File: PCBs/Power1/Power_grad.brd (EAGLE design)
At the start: 80.9 x 67.1 mm, 21 parts

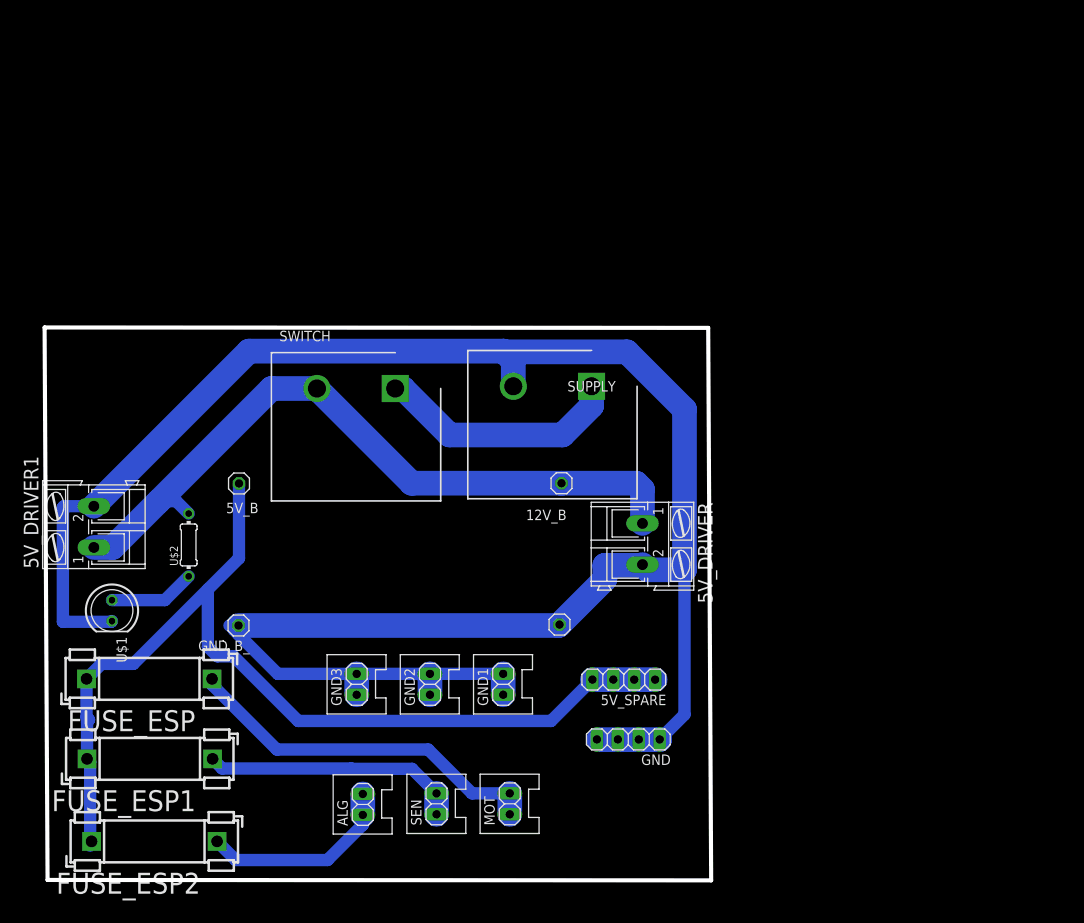
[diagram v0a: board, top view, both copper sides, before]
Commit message: Power modify
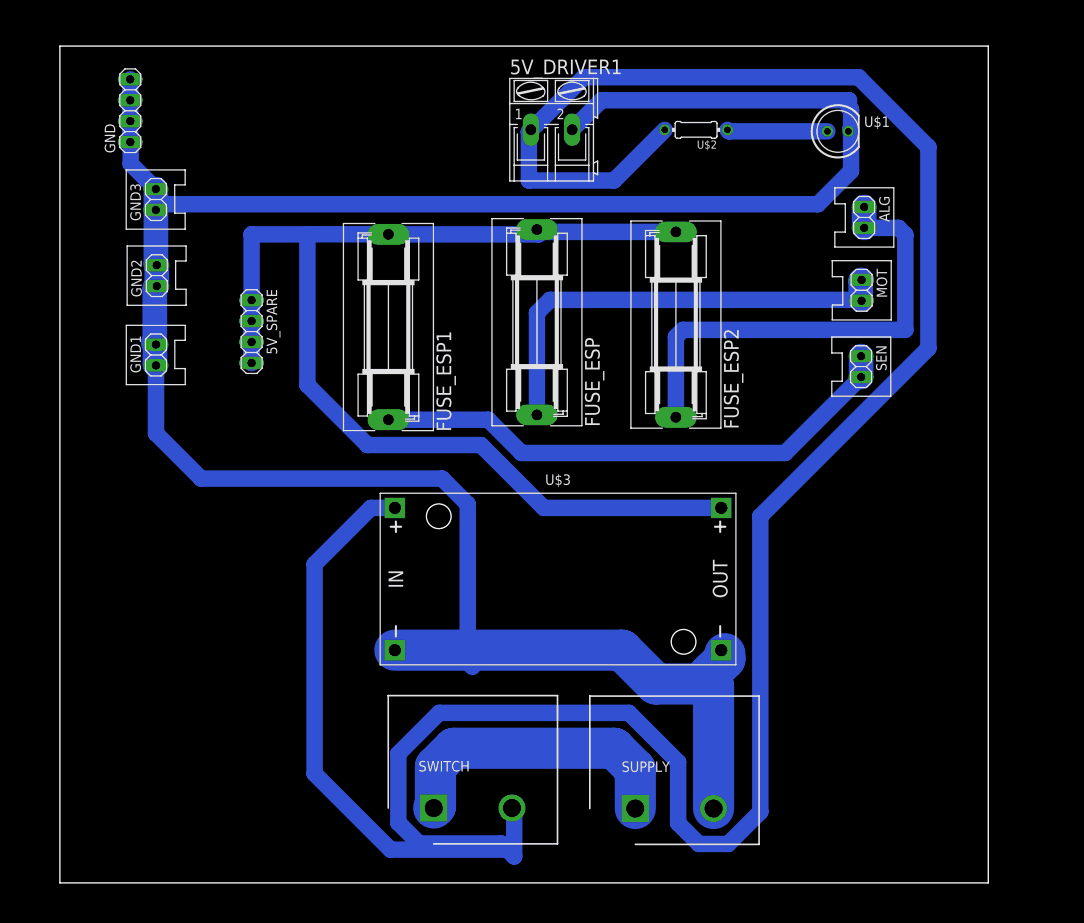
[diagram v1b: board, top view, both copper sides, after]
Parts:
- removed 12V_B, 5V_B, GND_B, GND_B_: (no value), ALL:1X01
- removed 5V_DRIVER: (no value), ALL:AK300/2
- added U$3: DC-DC-STEP-DOWN-LM2596, ALL:DC-DC-STEP-DOWN-LM2596
- FUSE_ESP, FUSE_ESP1, FUSE_ESP2: value FUSEBLANK_5X20MM -> (none); device fuse:FUSE_HOLDER_5X20MM -> ALL:SH22,5A
- moved U$1 105.6 mm to (94.4, 91.2), turned to 0 degrees
- moved GND 97.4 mm to (8.54, 93.7), turned to 90 degrees
- moved ALG 93.7 mm to (97.6, 80.8), turned to 270 degrees
- moved FUSE_ESP2 83.9 mm to (74.8, 67.8), turned to 90 degrees
- moved U$2 79.6 mm to (77.2, 91.4), turned to 180 degrees
- moved MOT 75.6 mm to (97.3, 71.9), turned to 270 degrees
- moved SEN 74.0 mm to (97.3, 62.7), turned to 270 degrees
- moved 5V_DRIVER1 73.6 mm to (59.7, 91.4), turned to 0 degrees
- moved GND3 63.7 mm to (11.7, 83.0)
- moved 5V_SPARE 61.9 mm to (23.3, 66.9), turned to 270 degrees
- moved GND2 59.7 mm to (11.8, 73.7)
- moved FUSE_ESP 58.6 mm to (57.9, 68.1), turned to 90 degrees
- moved GND1 58.1 mm to (11.7, 64.1)
- moved FUSE_ESP1 56.6 mm to (39.9, 67.5), turned to 90 degrees
- moved SUPPLY 51.5 mm to (69.8, 9.03), turned to 0 degrees
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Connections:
- net 12V: now also U$3.IN+; no longer 12V_B.1, 5V_DRIVER.1
- net 5V: now also U$3.OUT+; no longer 5V_B.1
- net GND: now also U$3.IN-, U$3.OUT-; no longer 5V_DRIVER.2, GND_B.1, GND_B_.1
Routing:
- net 12V: track 88.0 -> 323.1 mm
- net SEN: track 31.5 -> 65.4 mm
- net GND: track 263.2 -> 296.5 mm
- net ALG: track 24.1 -> 57.4 mm
- net 5V: track 121.6 -> 150.1 mm
- net MOT: track 44.9 -> 55.0 mm
- net 12V_IN: track 30.0 -> 36.1 mm
- net N$1: track 10.5 -> 12.2 mm
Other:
- board size 80.9 x 67.1 mm -> 112.7 x 101.6 mm

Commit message: PID v1.0
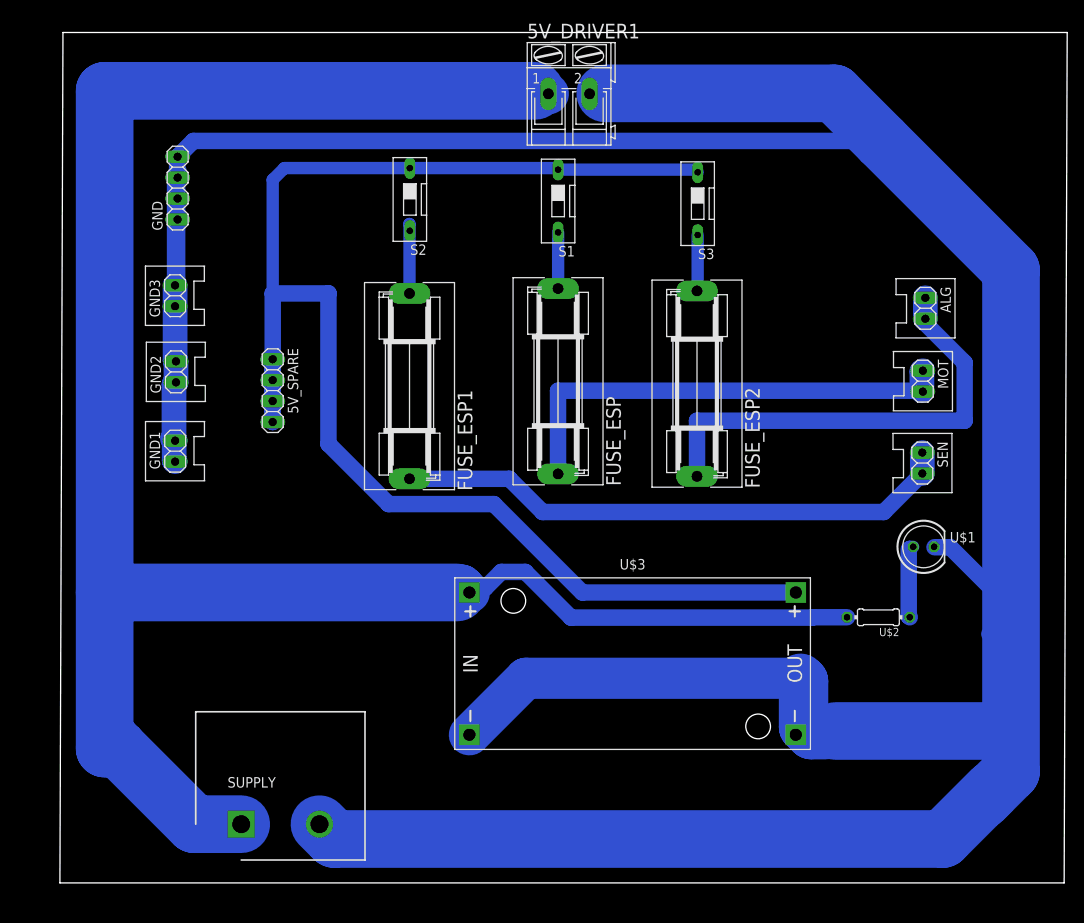
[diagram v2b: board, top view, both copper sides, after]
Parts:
- removed SWITCH: HB9500-9.5-2P, HB9500-9.5-2P:SHDR2W140P0X950_1X2_2055X1800X
- added S1, S2, S3: (no value), ALL:DS-01
- moved U$2 63.2 mm to (99.4, 32.2)
- moved U$1 51.5 mm to (104.8, 40.8)
- moved SUPPLY 47.9 mm to (22.0, 7.13)
- moved SEN 13.9 mm to (104.7, 51.0)
- moved U$3 13.7 mm to (69.5, 26.6)
- moved ALG 13.3 mm to (105.1, 69.8)
- moved MOT 13.3 mm to (104.8, 60.9)
- moved GND1 11.9 mm to (14.0, 52.4)
- moved GND2 11.9 mm to (14.1, 62.0)
- moved GND3 11.9 mm to (14.0, 71.3)
- moved GND 11.0 mm to (14.3, 84.3)
- moved 5V_SPARE 7.61 mm to (25.8, 59.8)
- moved FUSE_ESP2 7.61 mm to (77.3, 60.6)
- moved FUSE_ESP1 7.61 mm to (42.4, 60.3)
- moved FUSE_ESP 7.61 mm to (60.5, 60.9)
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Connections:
- removed net 12V_IN: SUPPLY.1, SWITCH.1
- new net N$2: FUSE_ESP1.2, S2.2
- new net N$3: FUSE_ESP.2, S1.2
- new net N$4: FUSE_ESP2.2, S3.2
- net 12V: now also SUPPLY.1; no longer SWITCH.2
- net 5V: now also S1.1, S2.1, S3.1; no longer FUSE_ESP.2, FUSE_ESP1.2, FUSE_ESP2.2
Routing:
- net GND: track 296.5 -> 454.6 mm
- net 12V: track 323.1 -> 264.1 mm
- net 12V_IN: track 36.1 -> 0.00 mm
- net 5V: track 150.1 -> 178.7 mm
- net N$2: track 0.00 -> 8.45 mm
- net N$3: track 0.00 -> 6.82 mm
- net N$4: track 0.00 -> 6.82 mm
- net N$1: track 12.2 -> 9.09 mm
- net SEN: track 65.4 -> 68.4 mm
- net MOT: track 55.0 -> 56.9 mm
- net ALG: track 57.4 -> 56.1 mm
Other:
- board size 112.7 x 101.6 mm -> 122.3 x 103.2 mm
